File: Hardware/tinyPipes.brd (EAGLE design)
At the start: 59.1 x 59 mm, 107 parts, among them Q1 CJ2302, Q2 CJ2302, Q3 CJ2302, Q4 BSS84, Q5 S9013, Q6 S9013, Q7 S9013, U1 TD1410, U2 ICS_V54_SIM900, U3 ATMEGA168MLF, U4 MAX4372, U5 SI4435POWER, U7 EEPROM-I2CSMD, X1 16mhz

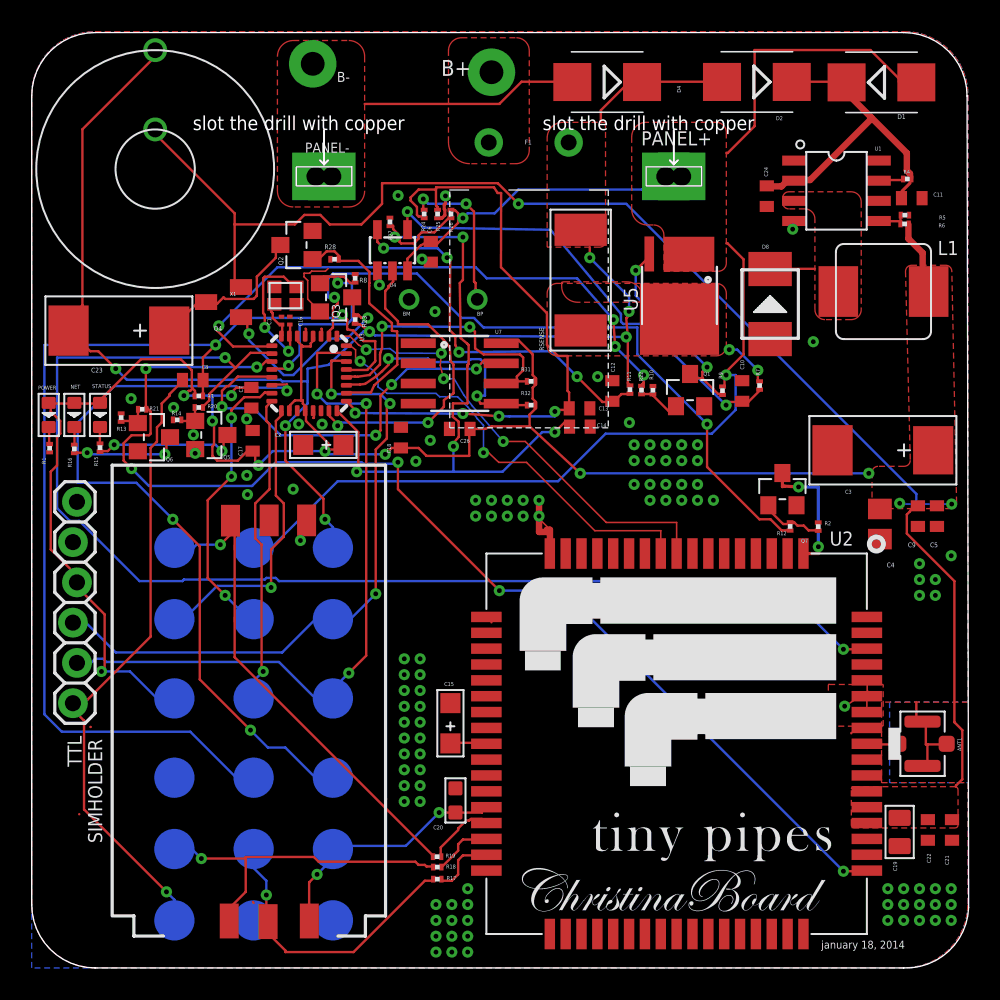
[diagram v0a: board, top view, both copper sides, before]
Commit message: stashing latest changes -- still a work in progress
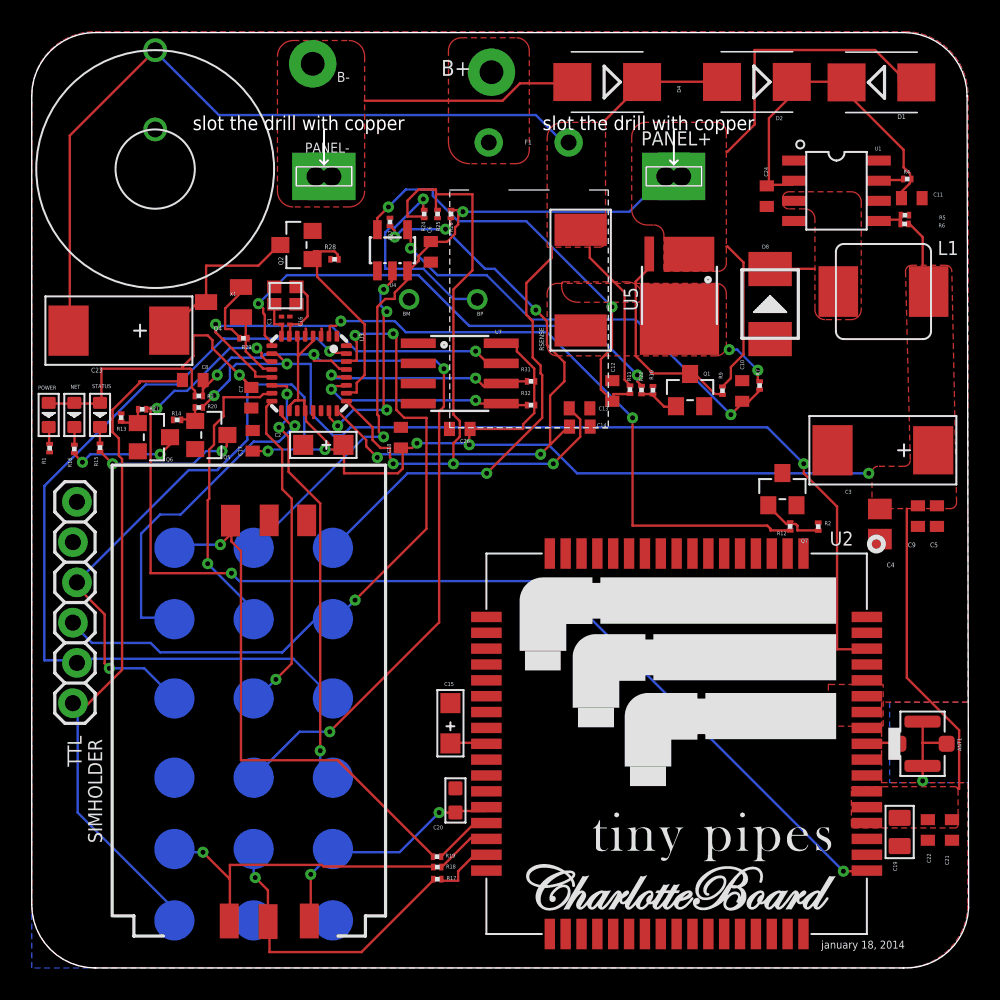
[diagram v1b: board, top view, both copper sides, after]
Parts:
- removed Q3: CJ2302, Discrete:SOT23
- removed R23, R8: 10k, rcl:R0201
- added R29: 10k, rcl:R0201
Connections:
- net LOW_SIDE renamed PILLOWTALK_LOW_SIDE
- removed net HIGH_SIDE: Q3.1, R8.2, U3.12
- removed net PFET_GATE: Q3.3, Q4.1, R23.1
- new net PILLOWTALK_HIGH_SIDE: Q4.1, R29.1, U3.12
- net BATTERY: no longer R23.2
- net GND: no longer Q3.2, R8.1
- net VCC: now also R29.2
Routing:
- net VCC: track 70.0 -> 4.25 mm, vias 3 -> 0
- net LTXD: track 29.3 -> 0.00 mm, vias 4 -> 0
- net LRXD: track 28.0 -> 0.00 mm, vias 2 -> 0
- net STATUS: track 82.0 -> 60.1 mm, vias 2 -> 3
- net LOAD_FET: track 48.2 -> 27.8 mm
- net GND: track 24.8 -> 6.96 mm, vias 107 -> 1
- net RST: track 67.8 -> 52.2 mm, vias 2 -> 4
- net PANEL: track 87.0 -> 72.7 mm
- net HIGH_SIDE: track 14.2 -> 0.00 mm, vias 2 -> 0
- net PFET_GATE: track 14.0 -> 0.00 mm, vias 2 -> 0
- net VROUTE: track 134.6 -> 146.1 mm, vias 9 -> 7
- net TX: track 44.9 -> 53.8 mm, vias 3 -> 1
- net PWRKEY: track 8.30 -> 0.00 mm, vias 2 -> 0
- net PANEL_VOLTAGE: track 45.8 -> 39.5 mm
- net PANEL_CURRENT: track 20.3 -> 14.2 mm, vias 2 -> 4
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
